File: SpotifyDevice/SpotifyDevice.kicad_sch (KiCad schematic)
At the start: 3 parts, among them U1 ESP32-S3-WROOM-1, U2 CR2013-MI2120

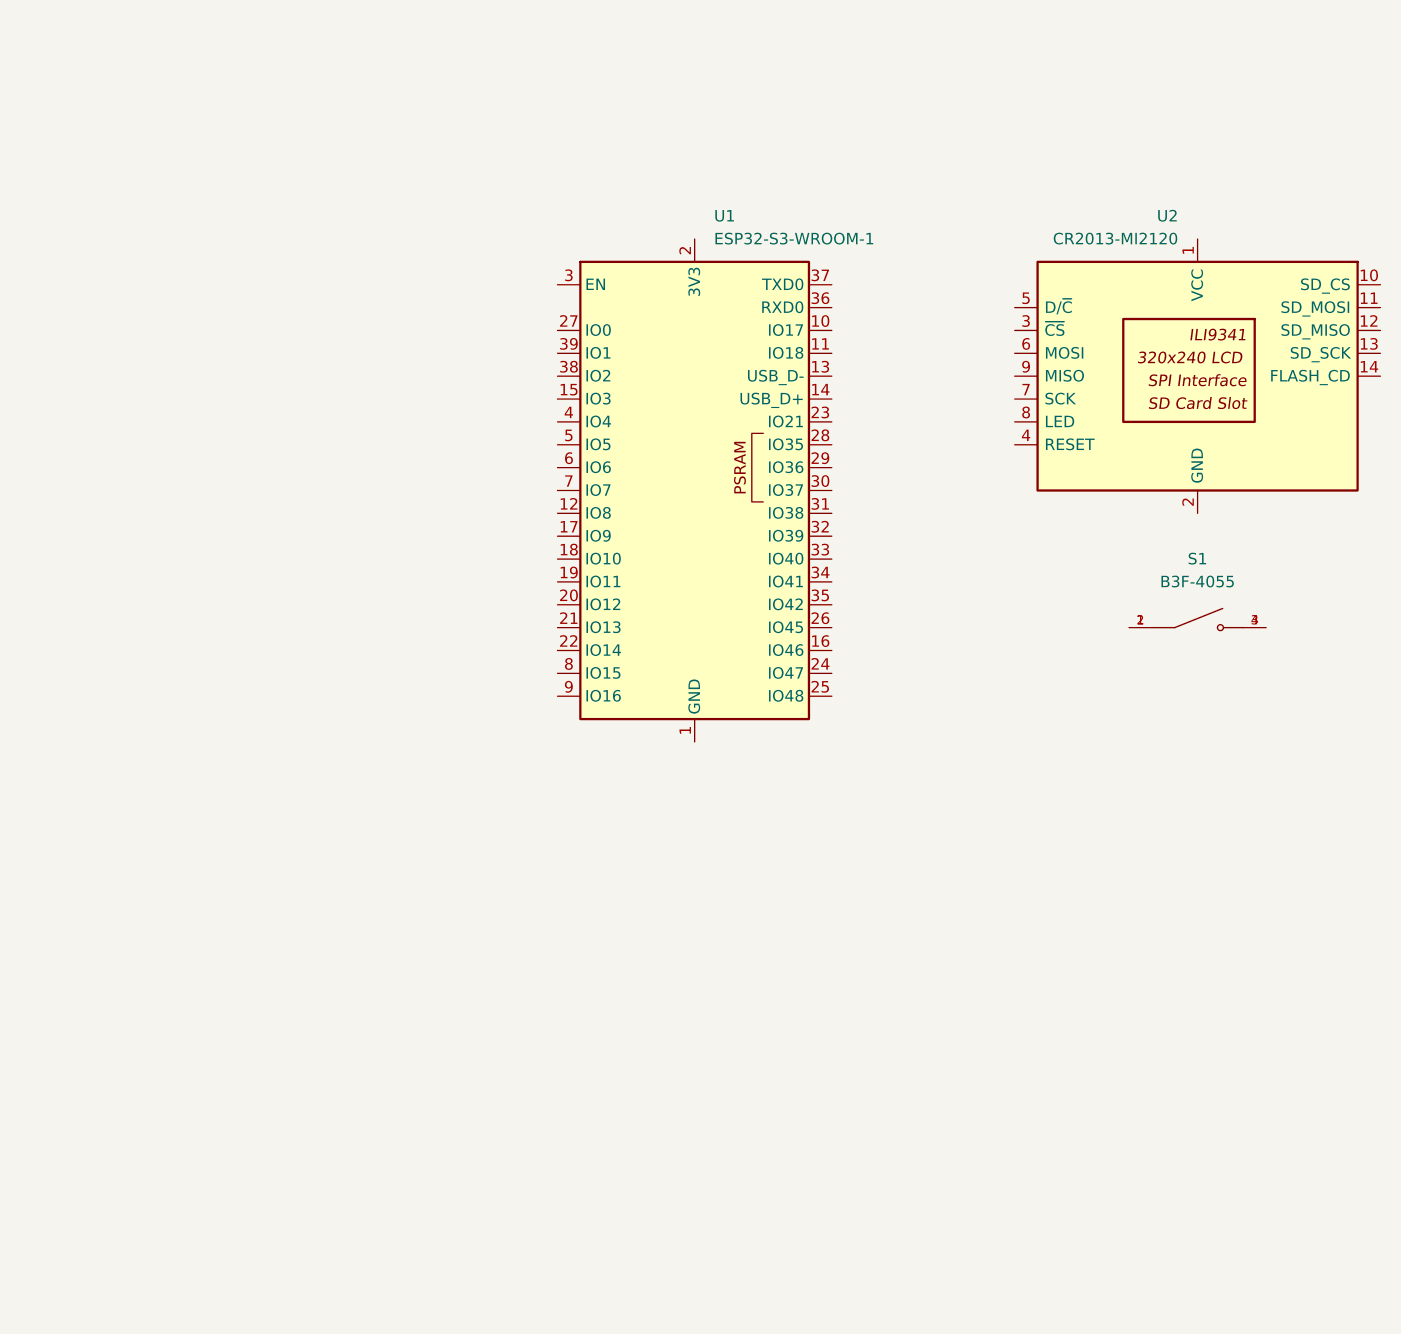
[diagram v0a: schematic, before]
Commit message: Draft 1 of Schematic Complete
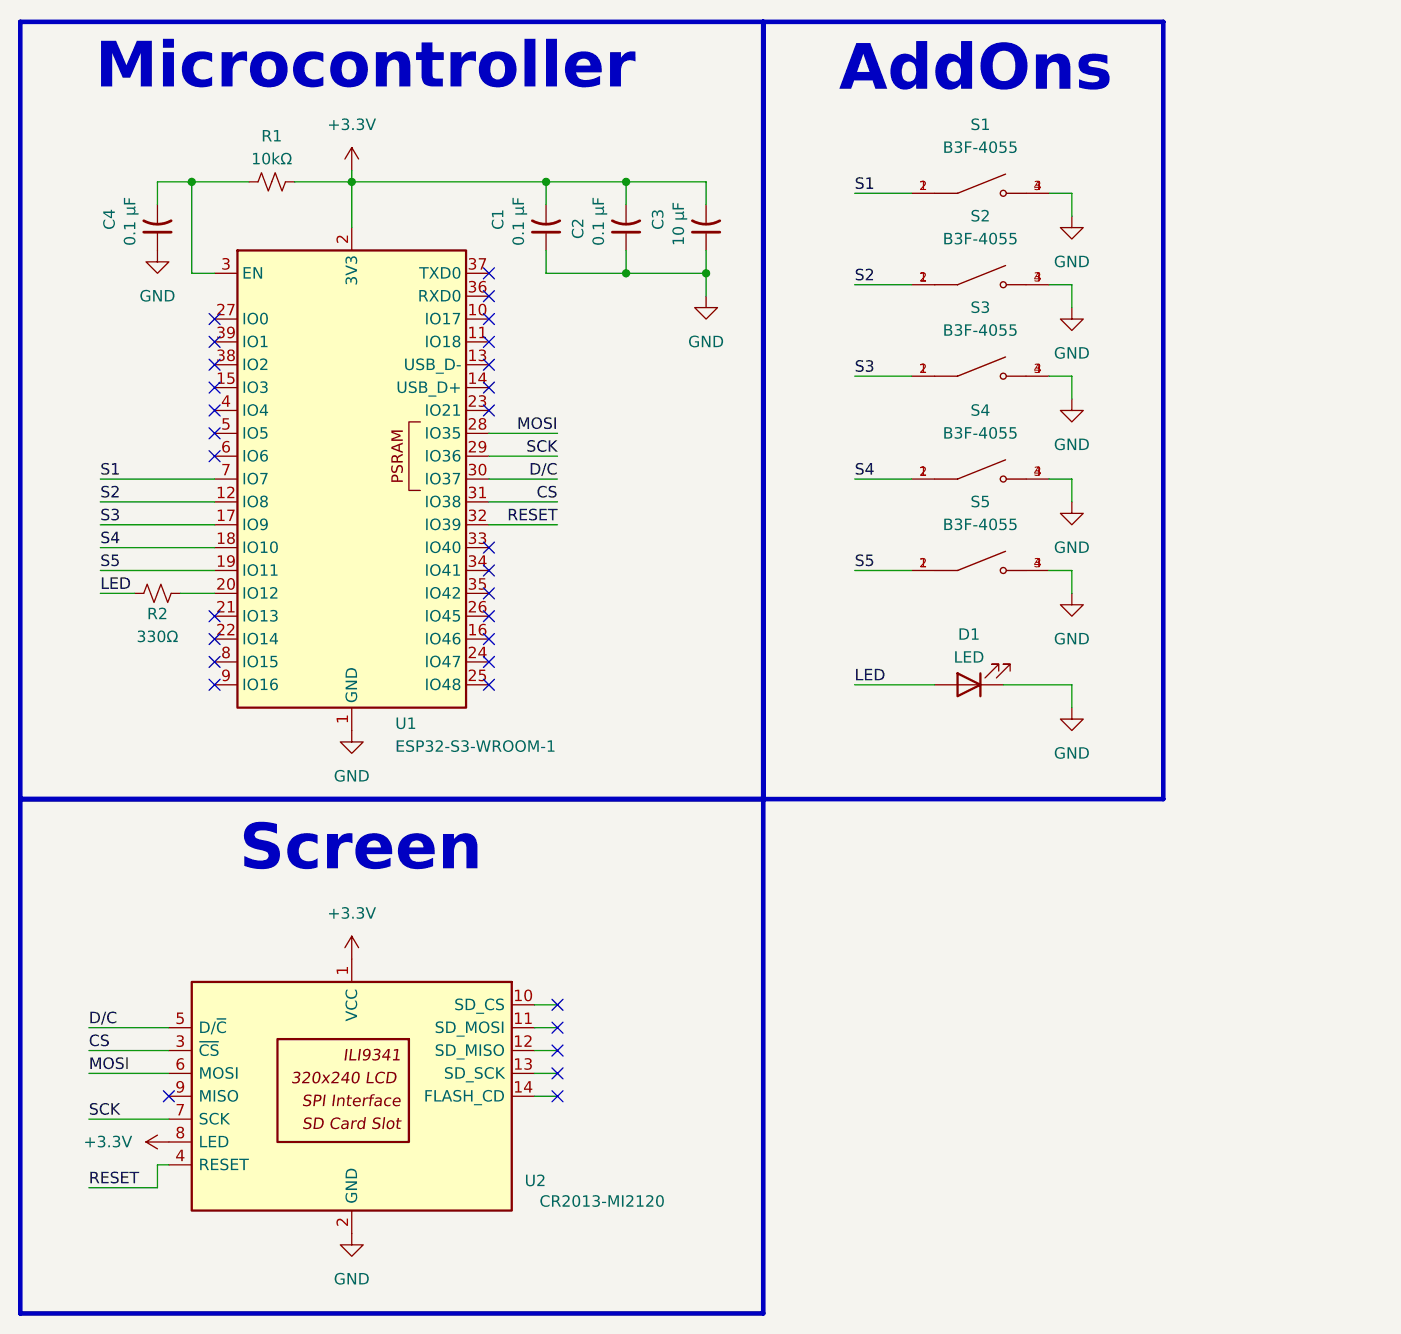
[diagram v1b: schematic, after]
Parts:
- added C1, C2, C4: 0.1 μF, symbol Device:C_Small_US
- added C3: 10 μF, symbol Device:C_Small_US
- added D1: LED, symbol Device:LED
- added R1: 10kΩ, symbol Device:R_Small_US
- added R2: 330Ω, symbol Device:R_Small_US
- added S2, S3, S4, S5: B3F-4055, ImportedParts:SW_B3F-4055, symbol Imported Parts:B3F-4055
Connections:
- net S1: now reaches S1.1, S1.2
- net S1: now also U1.7 (IO7)
- net GND: now reaches S1.3, S1.4
- net GND: now also U1.1 (GND), U1.40 (GND), U1.41 (GND), U2.2 (GND), C1.1, C2.1, C3.1, C4.1, D1.1 (K), S2.3, S2.4, S3.3, S3.4, S4.3, S4.4, S5.3, S5.4
- net S2: now reaches U1.12 (IO8)
- net S2: now also S2.1, S2.2
- net S3: now reaches U1.17 (IO9)
- net S3: now also S3.1, S3.2
- net S4: now reaches U1.18 (IO10)
- net S4: now also S4.1, S4.2
- net S5: now reaches U1.19 (IO11)
- net S5: now also S5.1, S5.2
- net +3.3V: now reaches U1.2 (3V3)
- net +3.3V: now also U2.1 (VCC), U2.8 (LED), C1.2, C2.2, C3.2, R1.2
- net at U1.20 (IO12): now also R2.2
- net MOSI: now reaches U1.28 (IO35)
- net MOSI: now also U2.6 (MOSI)
- net SCK: now reaches U1.29 (IO36)
- net SCK: now also U2.7 (SCK)
- net at U1.3 (EN): now also C4.2, R1.1
- net D/C: now reaches U1.30 (IO37)
- net D/C: now also U2.5 (D/~{C})
- net CS: now reaches U1.31 (IO38)
- net CS: now also U2.3 (~{CS})
- net RESET: now reaches U1.32 (IO39)
- net RESET: now also U2.4 (RESET)
- new net LED: D1.2 (A), R2.1
- no-connect marks 0 -> 31
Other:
- note added: "AddOns"
- note added: "Microcontroller"
- note added: "Screen"
- moved on the sheet: S1, U1, U2
